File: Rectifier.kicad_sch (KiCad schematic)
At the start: 0 parts

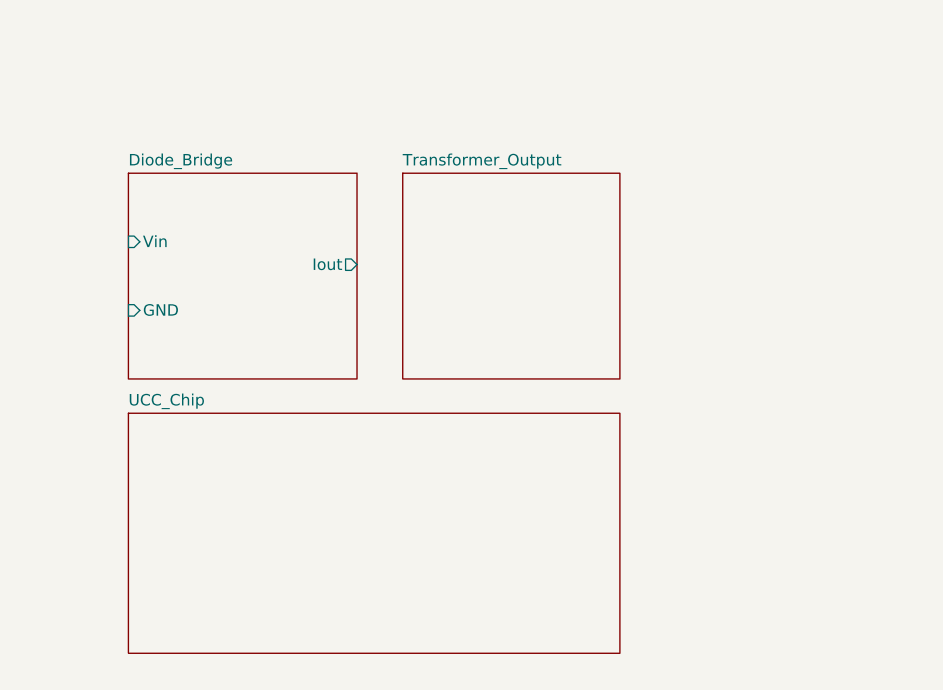
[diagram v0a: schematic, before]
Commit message: Added sheet pins
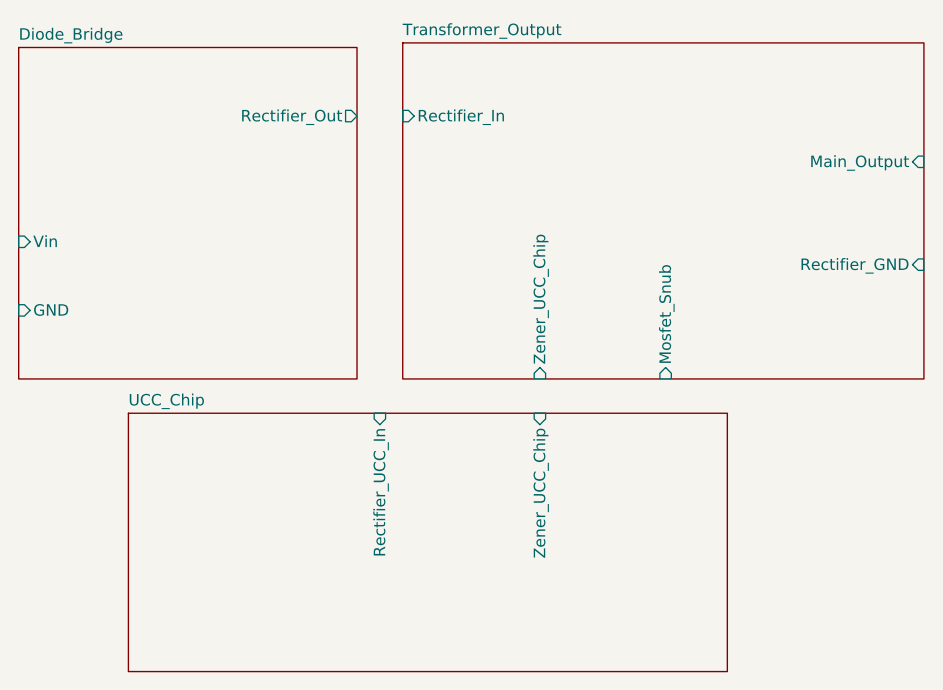
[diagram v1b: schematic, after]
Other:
- sheet Diode_Bridge ports: added Rectifier_Out; removed Iout
- sheet Transformer_Output ports: added Main_Output, Mosfet_Snub, Rectifier_GND, Rectifier_In, Zener_UCC_Chip; removed none
- sheet UCC_Chip ports: added Rectifier_UCC_In, Zener_UCC_Chip; removed none
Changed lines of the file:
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@@
 	(sheet
 		(at 107.95 132.08)
-		(size 54.61 26.67)
+		(size 66.548 28.702)
 		(exclude_from_sim no)
 		(in_bom yes)
@@
 		)
 		(property "Sheetfile" "UCC_Chip.kicad_sch"
-			(at 107.95 159.3346 0)
+			(at 107.95 161.3666 0)
 			(hide yes)
 			(show_name no)
@@
 				)
 				(justify left top)
+			)
+		)
+		(pin "Rectifier_UCC_In" input
+			(at 135.89 132.08 90)
+			(effects
+				(font
+					(size 1.27 1.27)
+				)
+				(justify right)
+			)
+		)
+		(pin "Zener_UCC_Chip" input
+			(at 153.67 132.08 90)
+			(effects
+				(font
+					(size 1.27 1.27)
+				)
+				(justify right)
 			)
 		)
@@
 	)
 	(sheet
-		(at 107.95 105.41)
-		(size 25.4 22.86)
+		(at 95.758 91.44)
+		(size 37.592 36.83)
 		(exclude_from_sim no)
 		(in_bom yes)
@@
 		)
 		(property "Sheetname" "Diode_Bridge"
-			(at 107.95 104.6984 0)
+			(at 95.758 90.7284 0)
 			(show_name no)
 			(do_not_autoplace no)
@@
 		)
 		(property "Sheetfile" "Diode_Bridge.kicad_sch"
-			(at 107.95 128.8546 0)
+			(at 95.758 128.8546 0)
 			(hide yes)
 			(show_name no)
@@
 		)
 		(pin "GND" input
-			(at 107.95 120.65 180)
+			(at 95.758 120.65 180)
 			(effects
 				(font
@@
 		)
 		(pin "Vin" input
-			(at 107.95 113.03 180)
-			(effects
-				(font
-					(size 1.27 1.27)
-				)
-				(justify left)
-			)
-		)
-		(pin "Iout" output
-			(at 133.35 115.57 0)
+			(at 95.758 113.03 180)
+			(effects
+				(font
+					(size 1.27 1.27)
+				)
+				(justify left)
+			)
+		)
+		(pin "Rectifier_Out" output
+			(at 133.35 99.06 0)
 			(effects
 				(font
@@
 	)
 	(sheet
-		(at 138.43 105.41)
-		(size 24.13 22.86)
+		(at 138.43 90.932)
+		(size 57.912 37.338)
 		(exclude_from_sim no)
 		(in_bom yes)
@@
 		)
 		(property "Sheetname" "Transformer_Output"
-			(at 138.43 104.6984 0)
+			(at 138.43 90.2204 0)
 			(show_name no)
 			(do_not_autoplace no)
@@
 			)
 		)
+		(pin "Mosfet_Snub" input
+			(at 167.64 128.27 270)
+			(effects
+				(font
+					(size 1.27 1.27)
+				)
+				(justify left)
+			)
+		)
+		(pin "Rectifier_In" input
+			(at 138.43 99.06 180)
+			(effects
+				(font
+					(size 1.27 1.27)
+				)
+				(justify left)
+			)
+		)
+		(pin "Zener_UCC_Chip" input
+			(at 153.67 128.27 270)
+			(effects
+				(font
+					(size 1.27 1.27)
+				)
+				(justify left)
+			)
+		)
+		(pin "Main_Output" input
+			(at 196.342 104.14 0)
+			(effects
+				(font
+					(size 1.27 1.27)
+				)
+				(justify right)
+			)
+		)
+		(pin "Rectifier_GND" input
+			(at 196.342 115.57 0)
+			(effects
+				(font
+					(size 1.27 1.27)
+				)
+				(justify right)
+			)
+		)
